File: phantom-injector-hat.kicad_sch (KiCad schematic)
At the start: 1 part, among them U1 LT8362EMSE-PBF

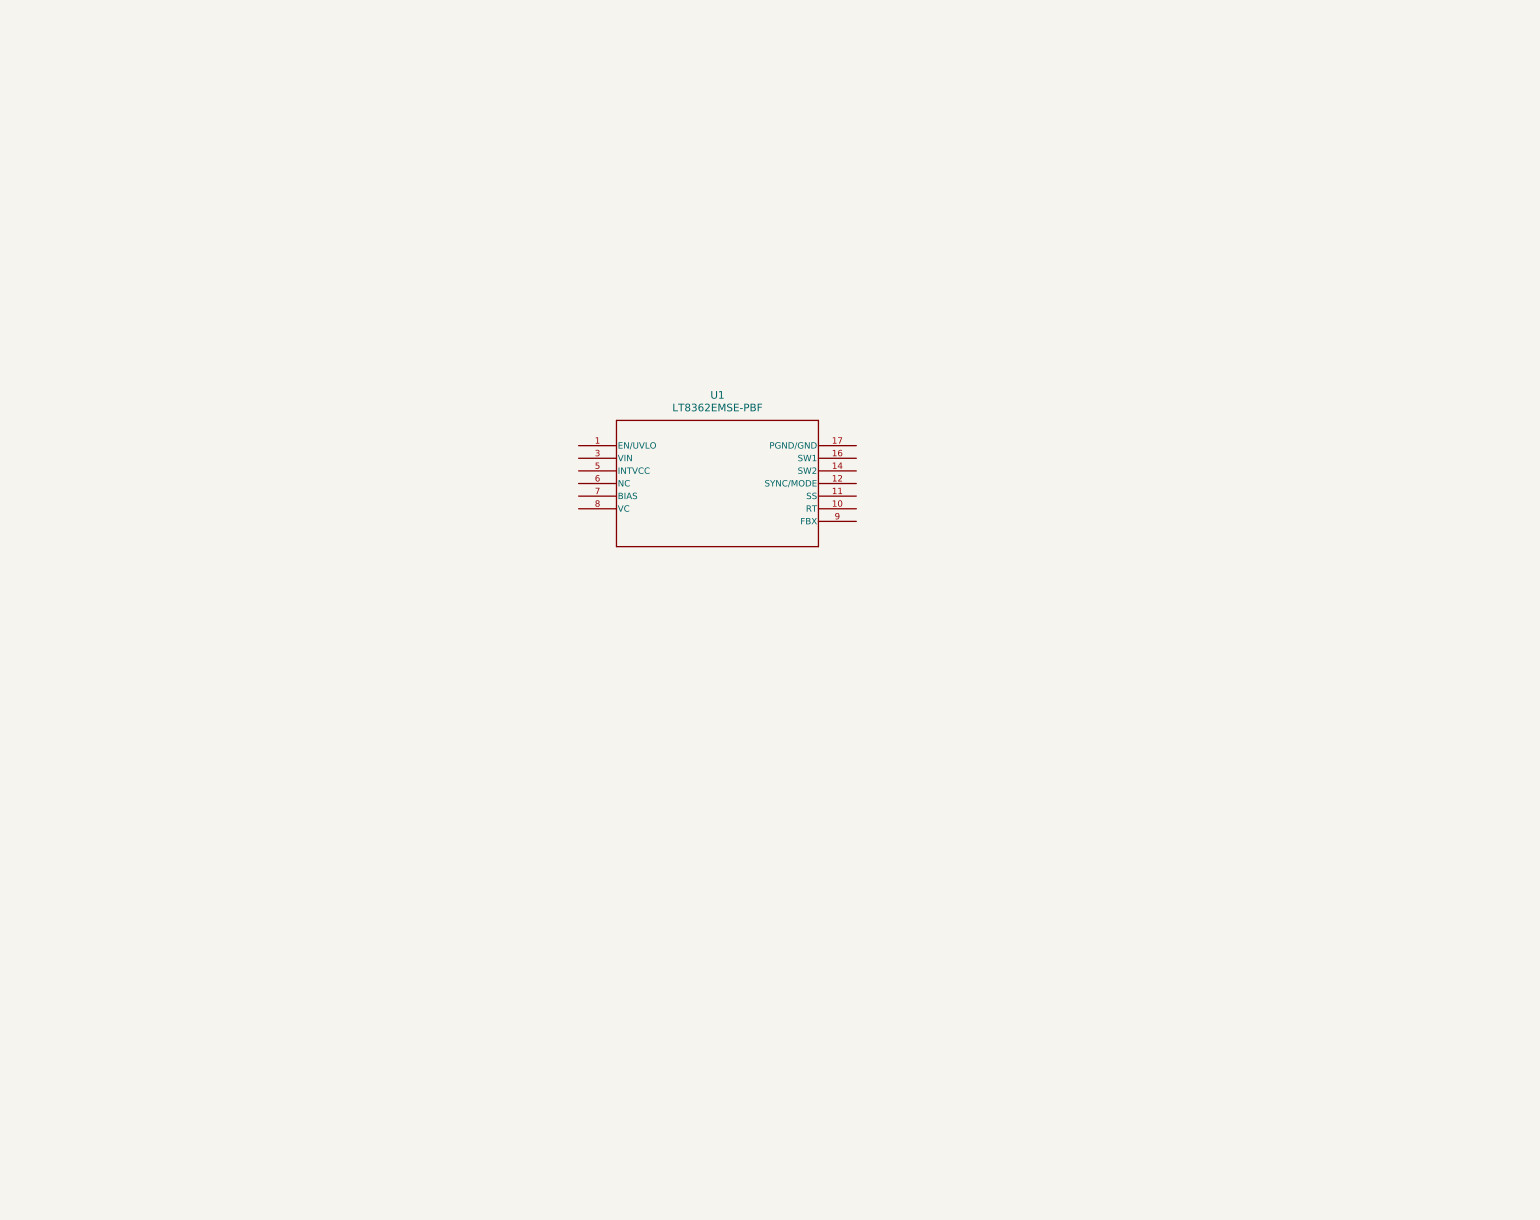
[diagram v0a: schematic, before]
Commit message: WIP
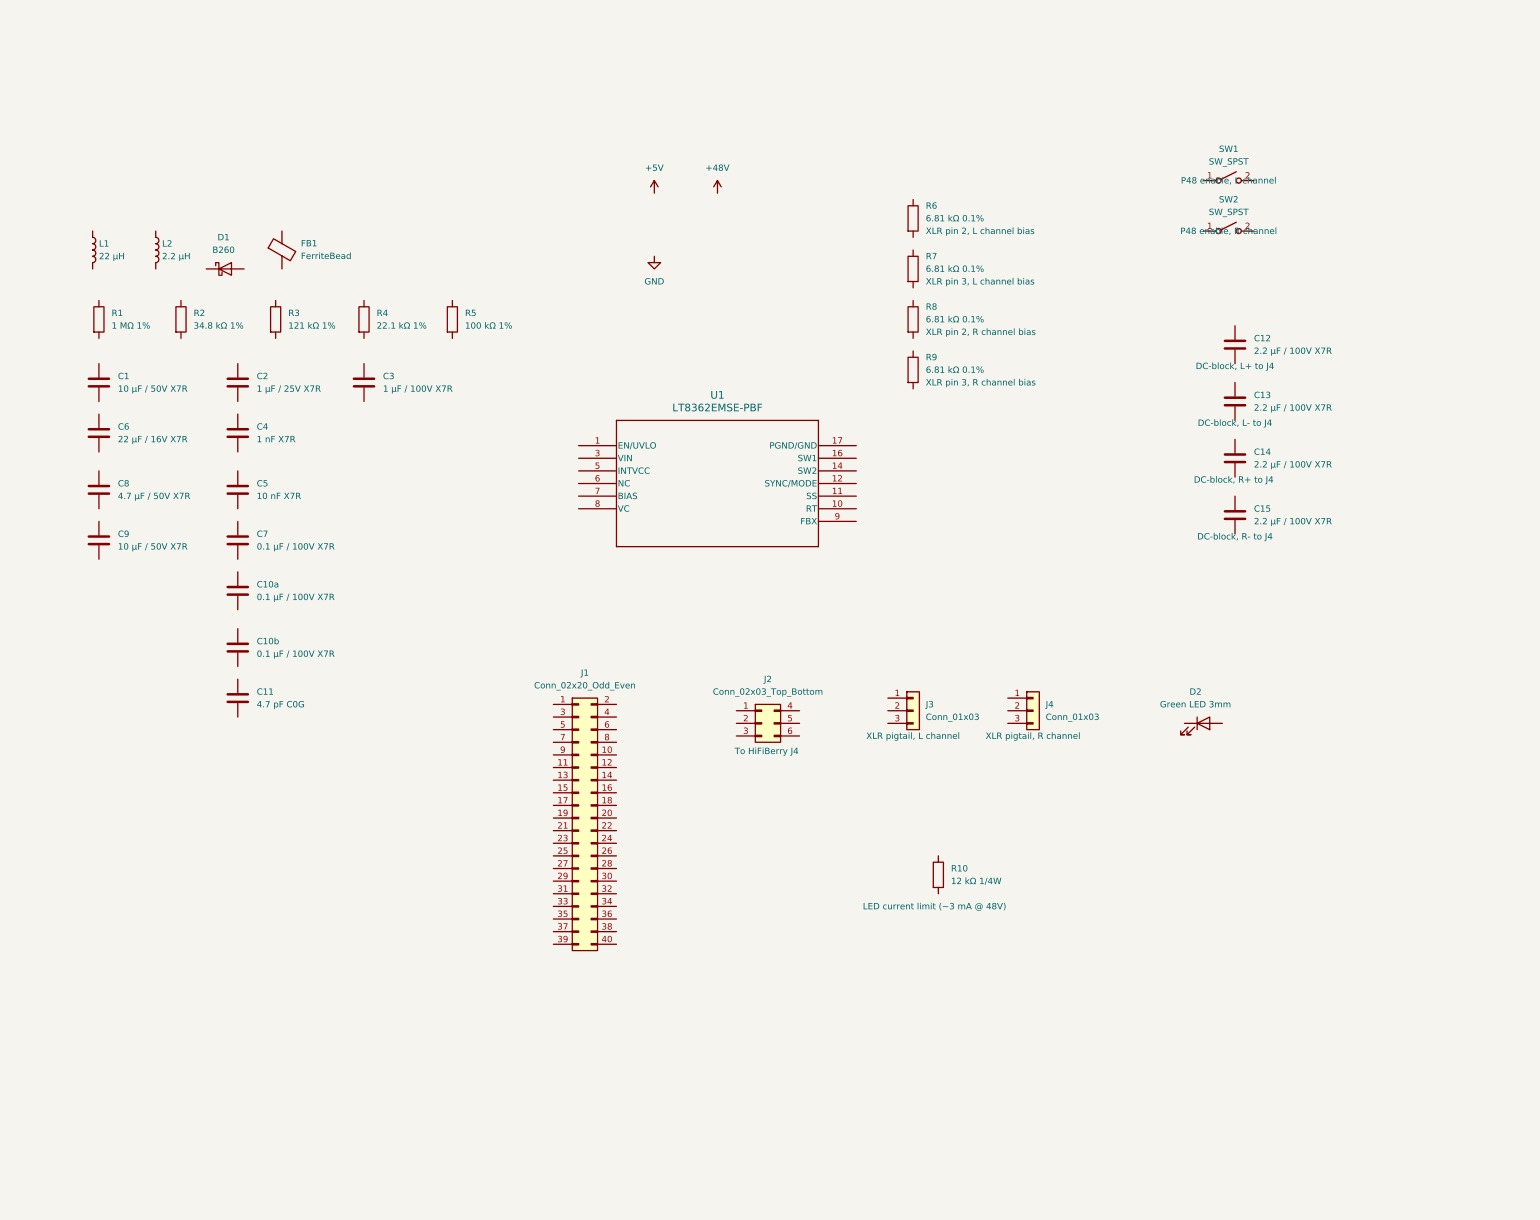
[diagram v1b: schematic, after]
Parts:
- added C1, C9: 10 µF / 50V X7R, Capacitor_SMD:C_1210_3225Metric_Pad1.33x2.70mm_HandSolder, symbol Device:C
- added C10a, C10b, C7: 0.1 µF / 100V X7R, Capacitor_SMD:C_0805_2012Metric_Pad1.18x1.45mm_HandSolder, symbol Device:C
- added C11: 4.7 pF C0G, Capacitor_SMD:C_0805_2012Metric_Pad1.18x1.45mm_HandSolder, symbol Device:C
- added C12, C13, C14, C15: 2.2 µF / 100V X7R, Capacitor_SMD:C_1812_4532Metric_Pad1.57x3.40mm_HandSolder, symbol Device:C
- added C2: 1 µF / 25V X7R, Capacitor_SMD:C_0805_2012Metric_Pad1.18x1.45mm_HandSolder, symbol Device:C
- added C3: 1 µF / 100V X7R, Capacitor_SMD:C_1206_3216Metric_Pad1.33x1.80mm_HandSolder, symbol Device:C
- added C4: 1 nF X7R, Capacitor_SMD:C_0805_2012Metric_Pad1.18x1.45mm_HandSolder, symbol Device:C
- added C5: 10 nF X7R, Capacitor_SMD:C_0805_2012Metric_Pad1.18x1.45mm_HandSolder, symbol Device:C
- added C6: 22 µF / 16V X7R, Capacitor_SMD:C_1210_3225Metric_Pad1.33x2.70mm_HandSolder, symbol Device:C
- added C8: 4.7 µF / 50V X7R, Capacitor_SMD:C_1210_3225Metric_Pad1.33x2.70mm_HandSolder, symbol Device:C
- added D1: B260, Diode_SMD:D_SMB, symbol Diode:B260
- added D2: Green LED 3mm, symbol Device:LED
- added FB1: FerriteBead, Inductor_SMD:L_1206_3216Metric_Pad1.22x1.90mm_HandSolder, symbol Device:FerriteBead
- added J1: Conn_02x20_Odd_Even, symbol Connector_Generic:Conn_02x20_Odd_Even
- added J2: Conn_02x03_Top_Bottom, symbol Connector_Generic:Conn_02x03_Top_Bottom
- added J3, J4: Conn_01x03, Connector_PinHeader_2.54mm:PinHeader_1x03_P2.54mm_Vertical_SMD_Pin1Left, symbol Connector_Generic:Conn_01x03
- added L1: 22 µH, Inductor_SMD:L_Coilcraft_XAL5030-XXX, symbol Device:L
- added L2: 2.2 µH, symbol Device:L
- added R1: 1 MΩ 1%, Resistor_SMD:R_0805_2012Metric_Pad1.20x1.40mm_HandSolder, symbol Device:R
- added R10: 12 kΩ 1/4W, Resistor_SMD:R_0805_2012Metric_Pad1.20x1.40mm_HandSolder, symbol Device:R
- added R2: 34.8 kΩ 1%, Resistor_SMD:R_0805_2012Metric_Pad1.20x1.40mm_HandSolder, symbol Device:R
- added R3: 121 kΩ 1%, Resistor_SMD:R_0805_2012Metric_Pad1.20x1.40mm_HandSolder, symbol Device:R
- added R4: 22.1 kΩ 1%, Resistor_SMD:R_0805_2012Metric_Pad1.20x1.40mm_HandSolder, symbol Device:R
- added R5: 100 kΩ 1%, Resistor_SMD:R_0805_2012Metric_Pad1.20x1.40mm_HandSolder, symbol Device:R
- added R6, R7, R8, R9: 6.81 kΩ 0.1%, Resistor_SMD:R_0805_2012Metric_Pad1.20x1.40mm_HandSolder, symbol Device:R
- added SW1, SW2: SW_SPST, symbol Switch:SW_SPST

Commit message: updates
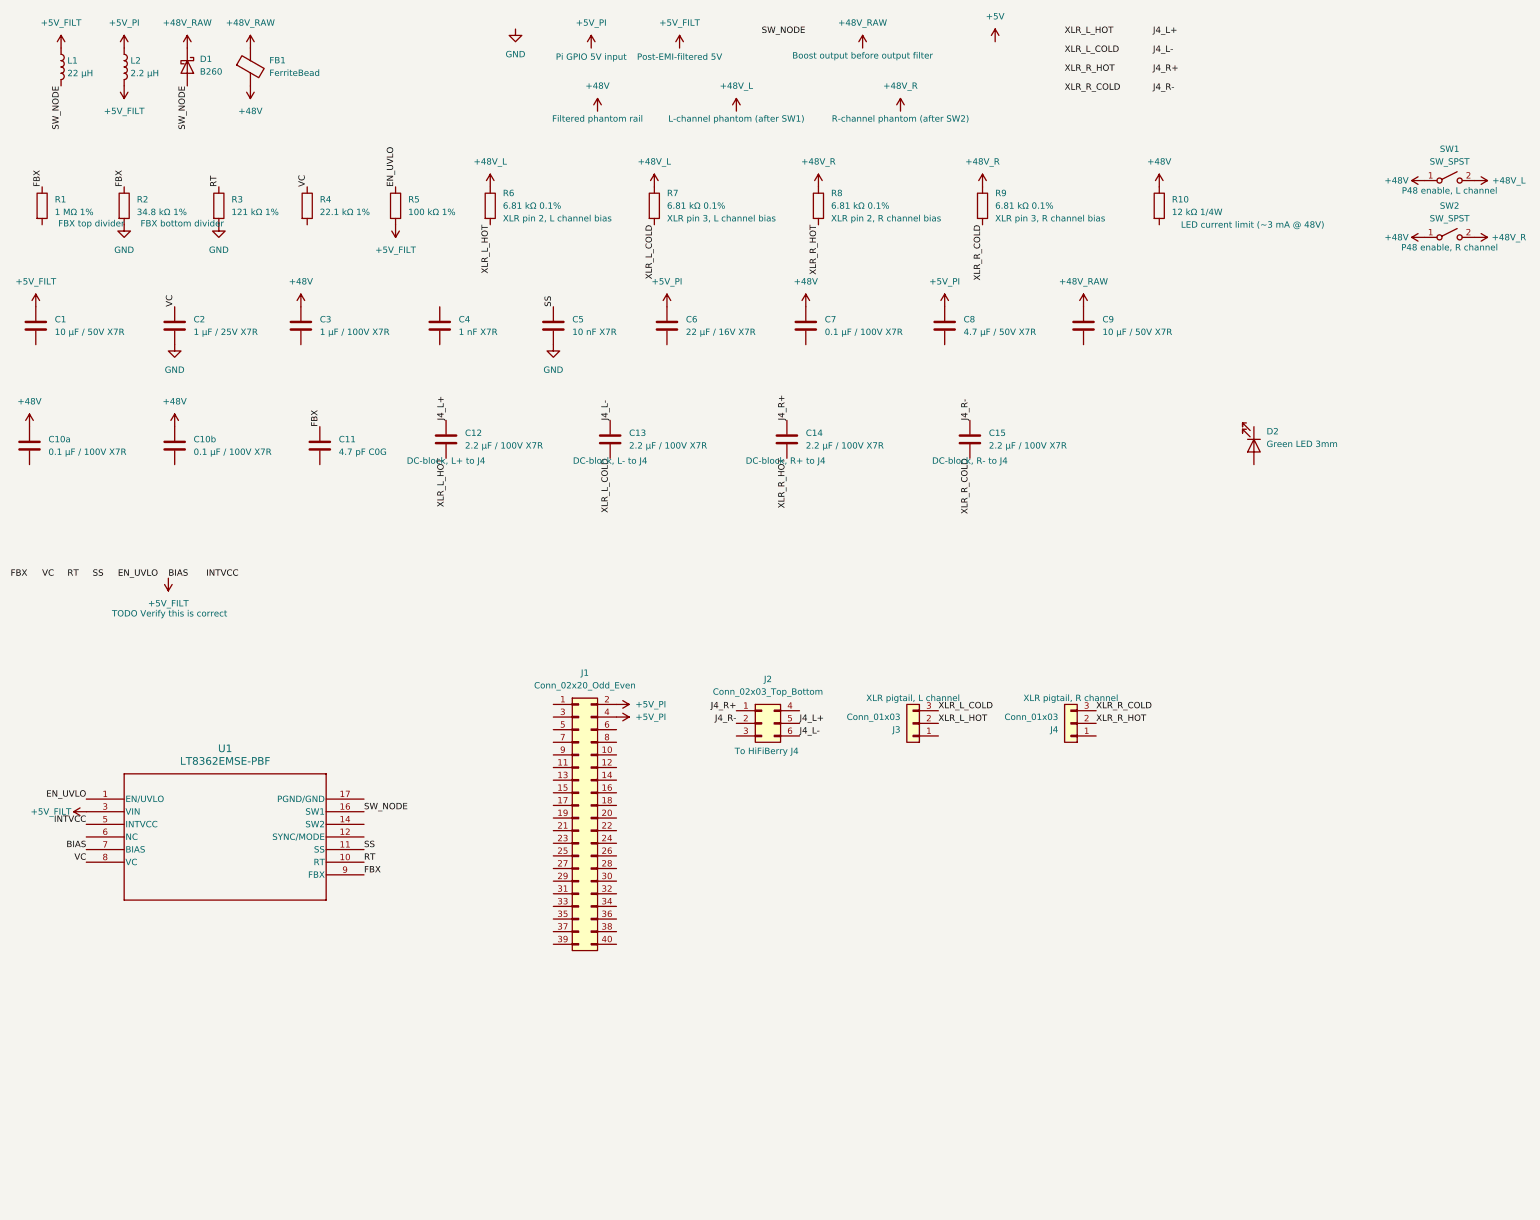
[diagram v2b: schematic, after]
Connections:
- net +48V: now also C10a.1, C10b.1, C3.1, C7.1, FB1.2, R10.1, SW1.1 (A), SW2.1 (A)
- net GND: now also C2.2, C5.2, R2.2, R3.2
- net +48V_RAW: now reaches FB1.1
- net +48V_RAW: now also C9.1, D1.1 (K)
- net RT: now reaches R3.1
- net RT: now also U1.10 (RT)
- net XLR_L_HOT: now reaches J3.2 (Pin_2)
- net XLR_L_HOT: now also C12.2, R6.2
- net XLR_L_COLD: now reaches J3.3 (Pin_3)
- net XLR_L_COLD: now also C13.2, R7.2
- net FBX: now reaches R1.1
- net FBX: now also C11.1, R2.1, U1.9 (FBX)
- net +5V_PI: now reaches C8.1
- net +5V_PI: now also C6.1, J1.2 (Pin_2), J1.4 (Pin_4), L2.1
- net +5V_FILT: now reaches L2.2
- net +5V_FILT: now also C1.1, L1.1, R5.2, U1.3 (VIN), U1.7 (BIAS)
- net J4_R+: now reaches C14.1
- net J4_R+: now also J2.1 (Pin_1)
- net XLR_R_HOT: now reaches C14.2
- net XLR_R_HOT: now also J4.2 (Pin_2), R8.2
- net J4_L+: now reaches C12.1
- net J4_L+: now also J2.5 (Pin_5)
- net EN_UVLO: now reaches R5.1
- net EN_UVLO: now also U1.1 (EN/UVLO)
- net VC: now reaches C2.1
- net VC: now also R4.1, U1.8 (VC)
- net +48V_L: now reaches SW1.2 (B)
- net +48V_L: now also R6.1, R7.1
- net +48V_R: now reaches R8.1
- net +48V_R: now also R9.1, SW2.2 (B)
- net J4_R-: now reaches J2.2 (Pin_2)
- net J4_R-: now also C15.1
- net J4_L-: now reaches J2.6 (Pin_6)
- net J4_L-: now also C13.1
- net XLR_R_COLD: now reaches R9.2
- net XLR_R_COLD: now also C15.2, J4.3 (Pin_3)
- net SW_NODE: now reaches D1.2 (A)
- net SW_NODE: now also L1.2, U1.16 (SW1)
- net SS: now reaches C5.1
- net SS: now also U1.11 (SS)
- net INTVCC: now reaches U1.5 (INTVCC)
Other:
- moved on the sheet: C1, C10a, C10b, C11, C12, C13, C14, C15, C2, C3, C4, C5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

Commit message: Wiring the schematic WIP
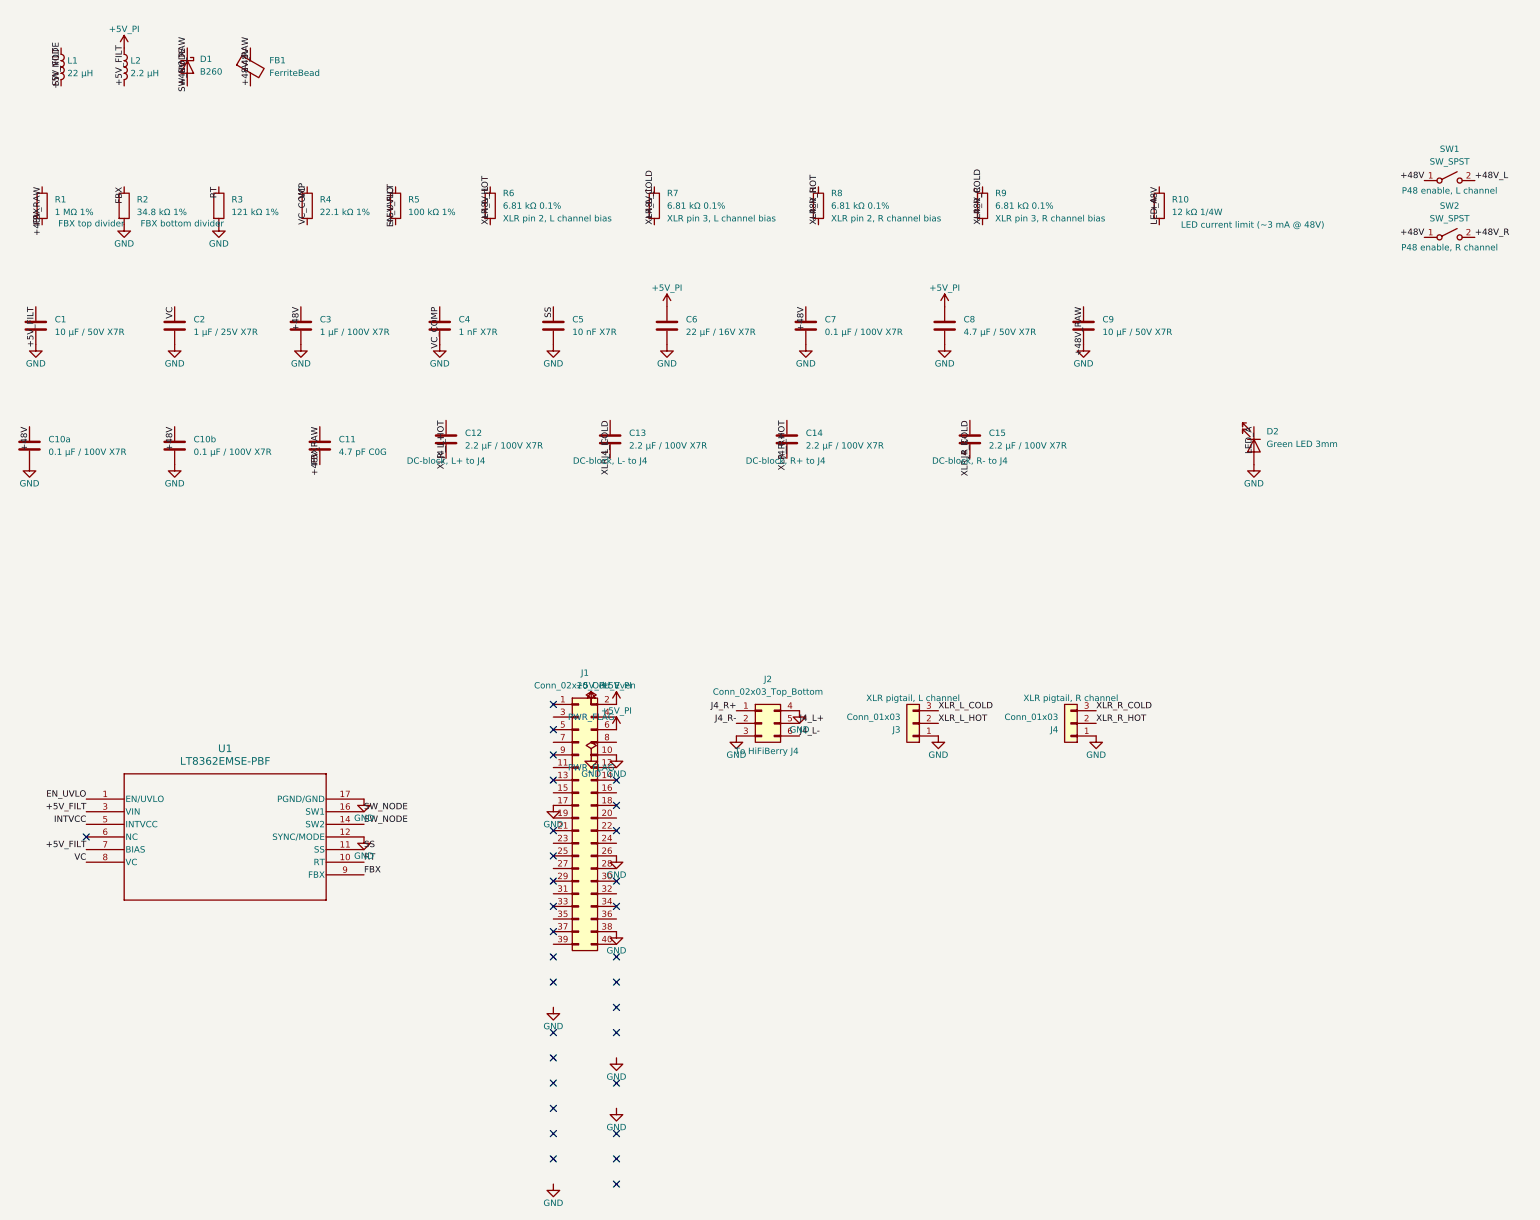
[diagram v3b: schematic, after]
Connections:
- net +48V: now also FB1.1; no longer FB1.2
- net +48V_RAW: now also C11.1, D1.2 (A), FB1.2, R1.1; no longer D1.1 (K), FB1.1
- net +5V_PI: now also J1.6 (Pin_6); no longer J1.4 (Pin_4)
- net FBX: now also C11.2, R1.2; no longer C11.1, R1.1
- net J4_L+: now also C12.2; no longer C12.1
- net J4_L-: now also C13.2; no longer C13.1
- net J4_R+: now also C14.2; no longer C14.1
- net J4_R-: now also C15.2; no longer C15.1
- net SW_NODE: now also D1.1 (K), U1.14 (SW2); no longer D1.2 (A)
- net XLR_L_COLD: now also C13.1; no longer C13.2
- net XLR_L_HOT: now also C12.1; no longer C12.2
- net XLR_R_COLD: now also C15.1; no longer C15.2
- net XLR_R_HOT: now also C14.1; no longer C14.2
- net VC_COMP: now reaches C4.1
- net VC_COMP: now also R4.2
- net LED_A: now reaches D2.1 (K)
- net LED_A: now also R10.2
- removed net GND: C2.2, C5.2, R2.2, R3.2
- no-connect marks 0 -> 31
